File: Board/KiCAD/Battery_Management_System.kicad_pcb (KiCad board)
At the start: 4 copper layers, 47.7 x 62.6 mm, 117 parts, among them J1 Conn_01x06_Socket, J10 Conn_01x02, J11 Conn_01x02, J12 Conn_01x02, J13 Conn_01x02, J2 Conn_ARM_SWD_TagConnect_TC2030, J4 Conn_01x03, J5 Conn_01x03, J7 Conn_01x05, J8 Conn_01x02, J9 Conn_01x02, Q1 AON7408, Q10 AON7407, Q2 AON7408, Q23 2N7002, Q24 2N7002, Q25 2N7002, Q26 2N7002, Q3 AON7408, Q4 AON7408, Q5 BSS83P, Q6 BSS83P, Q7 BSS83P, Q8 BSS83P, SW2 SW_Push, U1 BQ25730RSNR, U3 LTC2943CDD#PBF, U5 LMR50410, U6 INA219AxDCN, U7 INA219AxDCN, U8 INA219AxDCN, U9 STM32F103C8T6, Y1 Crystal_GND24_Small, Y4 CM8V-T1A-32.768KHZ-12.5PF-20P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

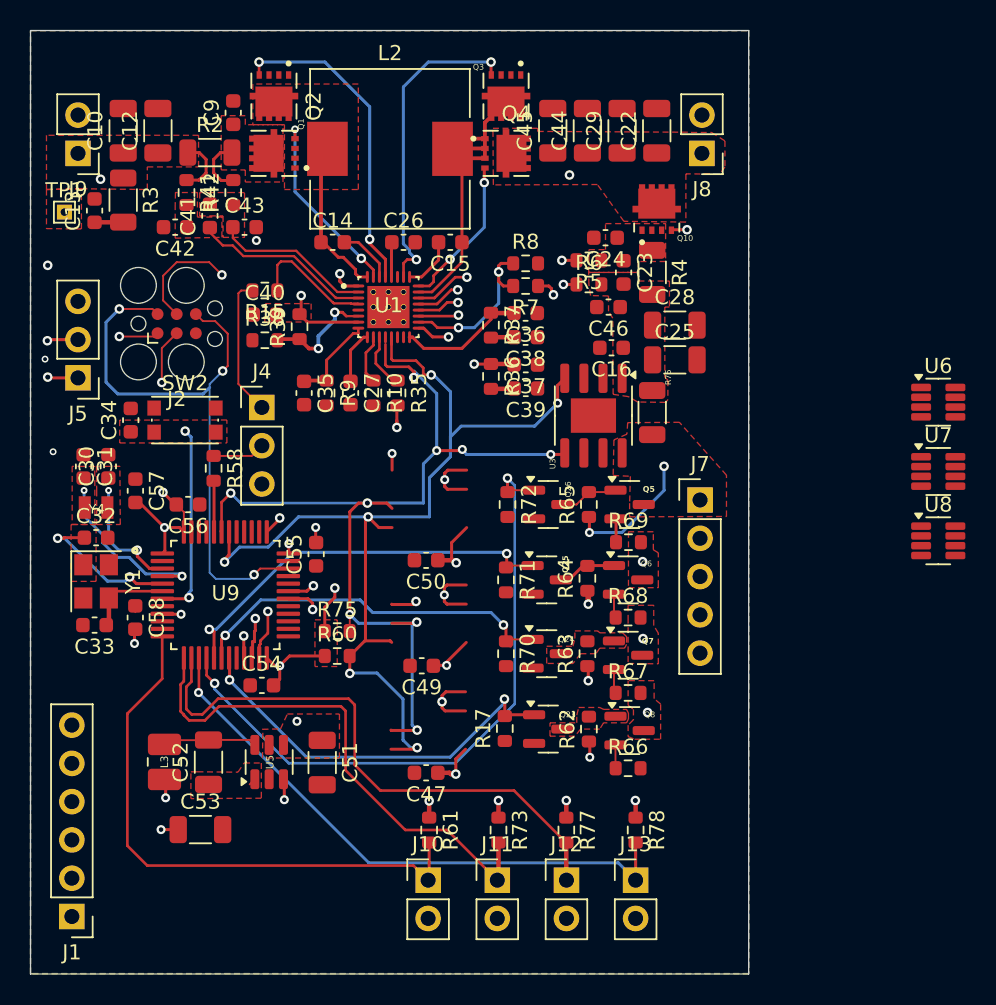
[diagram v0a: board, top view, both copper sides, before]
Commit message: finished PCB
PCB completed @andrewgreenberg
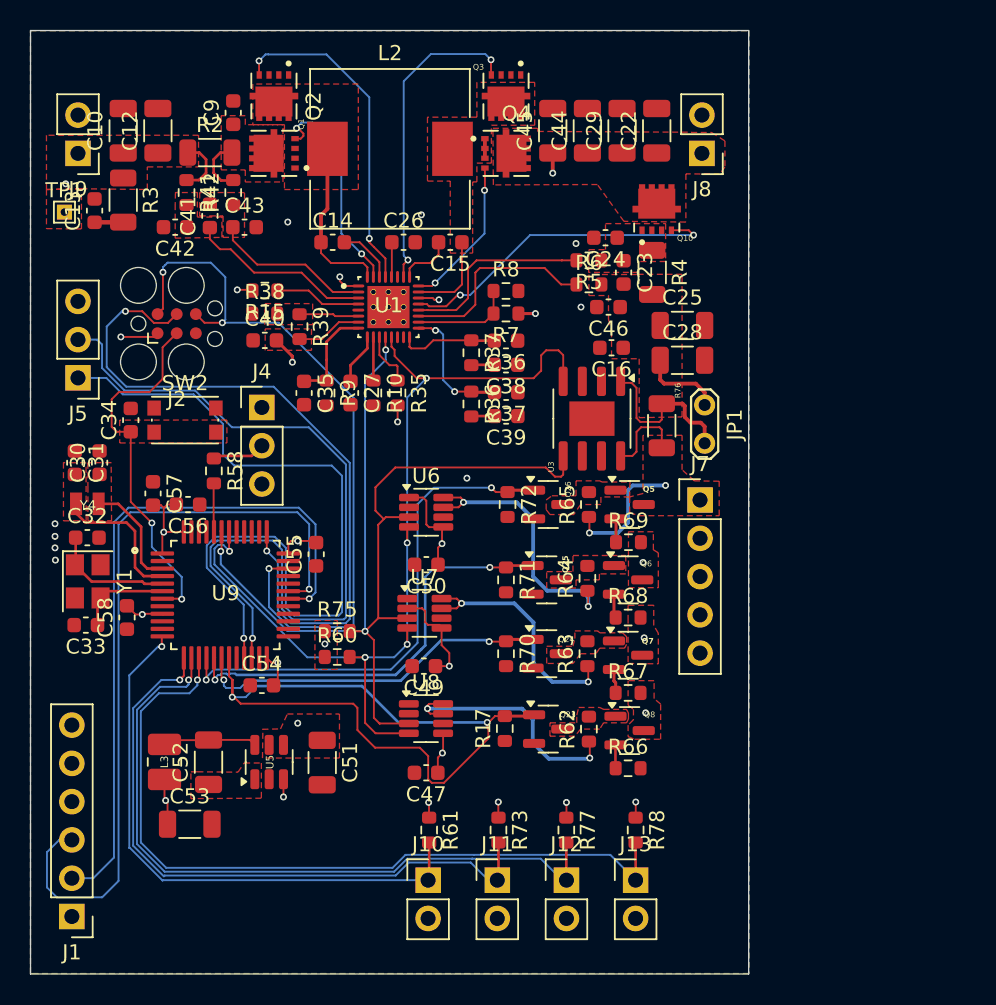
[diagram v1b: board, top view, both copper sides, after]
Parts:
- added JP1: Jumper_2_Bridged, TestPoint:TestPoint_2Pads_Pitch2.54mm_Drill0.8mm, F.Cu at (247.9, 71.5)
- moved U8 36.0 mm to (229.4, 92.3)
- moved U7 35.4 mm to (229.3, 85.3)
- moved U6 34.8 mm to (229.4, 78.6)
- moved C28 2.38 mm to (246.4, 68.5)
- moved C25 2.34 mm to (246.4, 66.2)
- moved R36 2.25 mm to (232.4, 71.4)
- moved R7 2.25 mm to (234.7, 65.4)
- moved C36 2.25 mm to (234.7, 67.2)
- moved C37 2.25 mm to (234.7, 70.7)
- moved C38 2.25 mm to (234.7, 68.8)
- moved C39 2.25 mm to (234.7, 72.2)
- moved R37 2.25 mm to (232.4, 68.0)
- moved R8 2.25 mm to (234.7, 63.9)
- moved R38 1.77 mm to (218.7, 65.4)
- moved C40 1.71 mm to (218.7, 67.2)
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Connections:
- C16 pad 1: Net-(U3-SENSE+) -> Net-(JP1-A)
- C23 pad 2: Net-(U3-SENSE+) -> Net-(JP1-A)
- C25 pad 1: Net-(U3-SENSE+) -> Net-(JP1-A)
- C28 pad 1: Net-(U3-SENSE+) -> Net-(JP1-A)
- C46 pad 1: Net-(U3-SENSE+) -> Net-(JP1-A)
- R4 pad 2: Net-(U3-SENSE+) -> Net-(JP1-A)
- R6 pad 2: Net-(U3-SENSE+) -> Net-(JP1-A)
- R76 pad 2: Net-(U3-SENSE+) -> Net-(JP1-B)
- U3 pad 1: Net-(U3-SENSE+) -> Net-(JP1-B)
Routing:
- net /Microcontroller/I2C2_SCL_To_Host: track 27.0 -> 52.8 mm, vias 2 -> 1
- net /Microcontroller/I2C2_SDA_To_Host: track 29.7 -> 55.1 mm, vias 2 -> 1
- net /Cell Interface/Cell_Balancer_1: track 26.9 -> 48.7 mm
- net SWCLK: track 26.5 -> 48.2 mm
- net 3.3V: track 62.8 -> 44.8 mm, vias 22 -> 17
- net /Microcontroller/Thermistor C4: track 39.9 -> 53.0 mm
- net Net-(U1-SW2): track 22.3 -> 9.47 mm
- net Net-(JP1-B): track 0.00 -> 11.3 mm
- net /Cell Interface/Cell_Balancer_4: track 43.8 -> 34.2 mm
- net /Charge Control/VBus: track 67.9 -> 77.2 mm
- net /Microcontroller/USART1_TX: track 37.2 -> 46.3 mm
- net SWDIO: track 40.0 -> 49.0 mm
- net VDDA: track 33.0 -> 25.0 mm
- net /Microcontroller/Thermistor C2: track 35.0 -> 43.0 mm, vias 0 -> 1
- net /Cell Interface/SDA: track 64.9 -> 71.9 mm, vias 9 -> 3
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- added copper zone on F.Cu, net Net-(JP1-A)
- added copper zone on F.Cu, net Net-(Q25-D)
- added copper zone on F.Cu, net Net-(Q26-D)
- added copper zone on F.Cu, net Net-(U1-ILIM_HIZ)
- added copper zone on F.Cu, net Net-(U1-SW2)
- removed copper zone on F.Cu, net Net-(U3-SENSE+)
- removed copper zone on F.Cu, net Net-(U9-PD0_OSC_IN)
